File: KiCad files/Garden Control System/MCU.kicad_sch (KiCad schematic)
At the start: 24 parts, among them SW1 SW_SPDT, U1 STM32F207ZGTx, Y1 16MHz

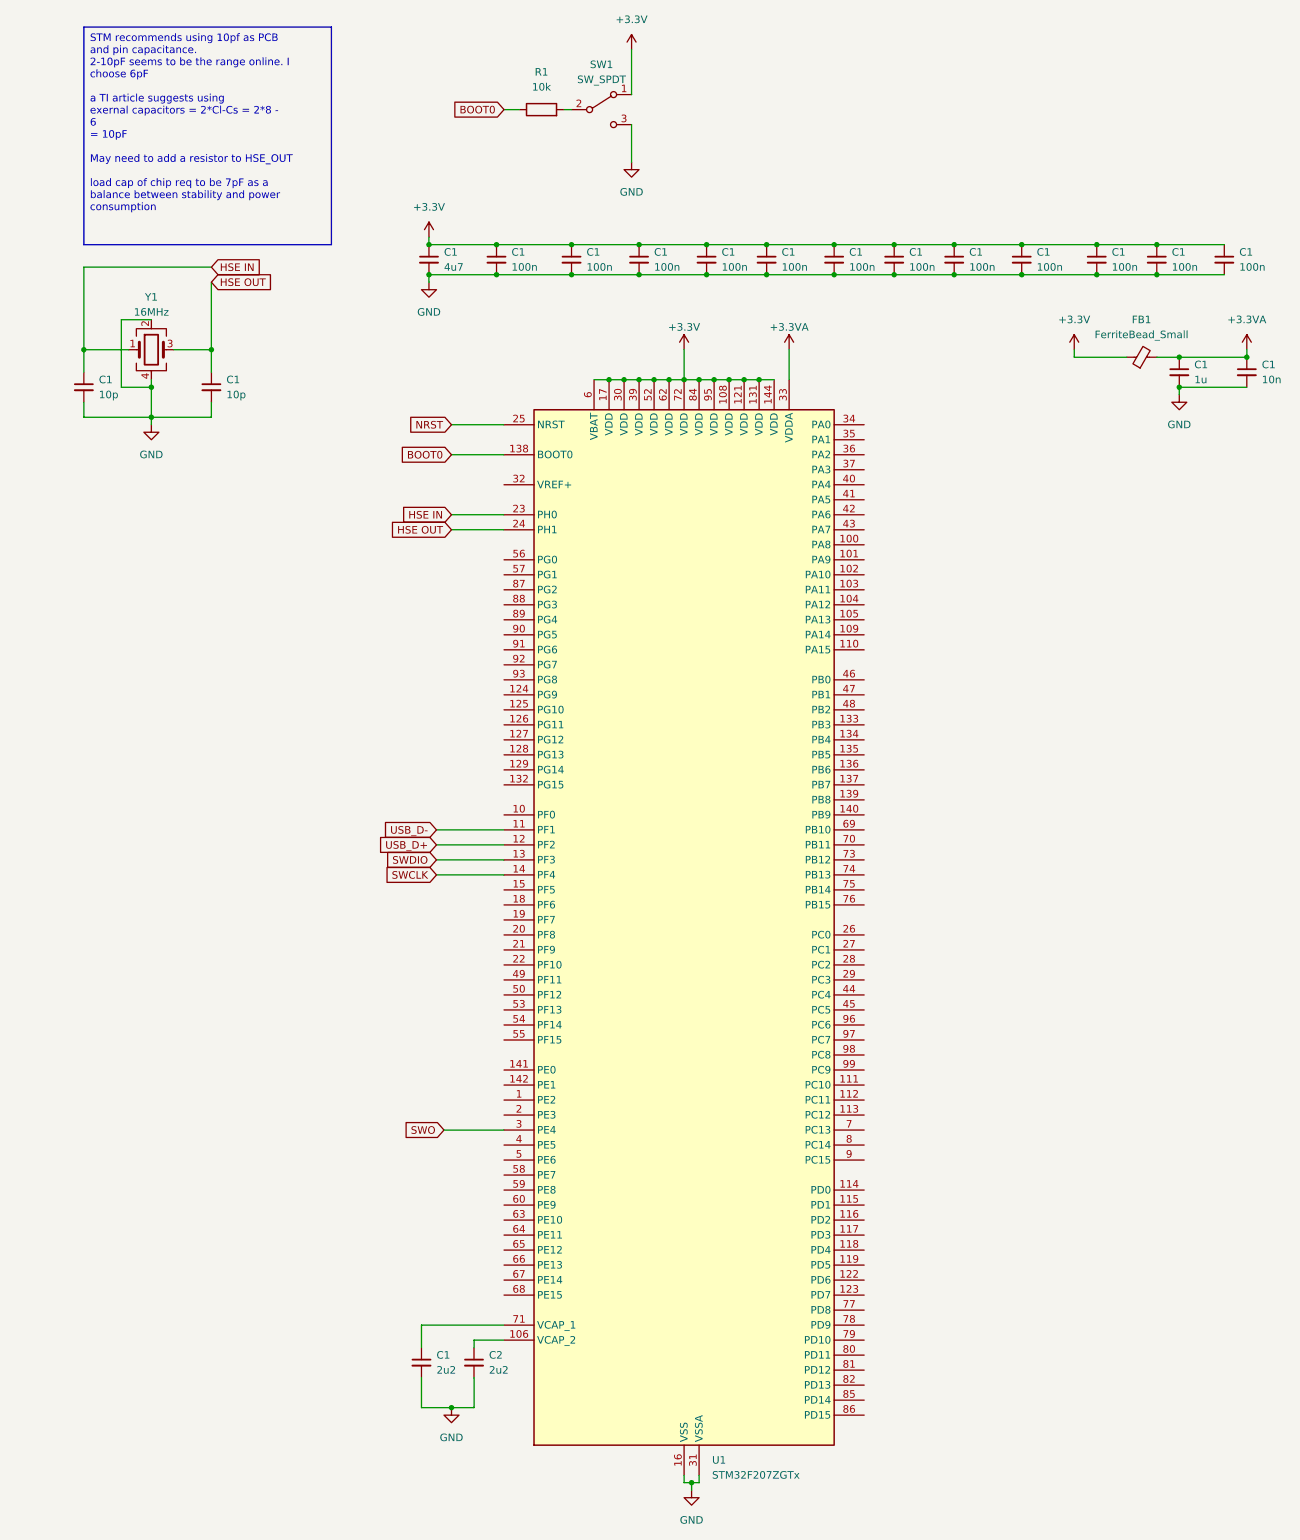
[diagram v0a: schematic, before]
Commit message: Close to finishing ethernet side
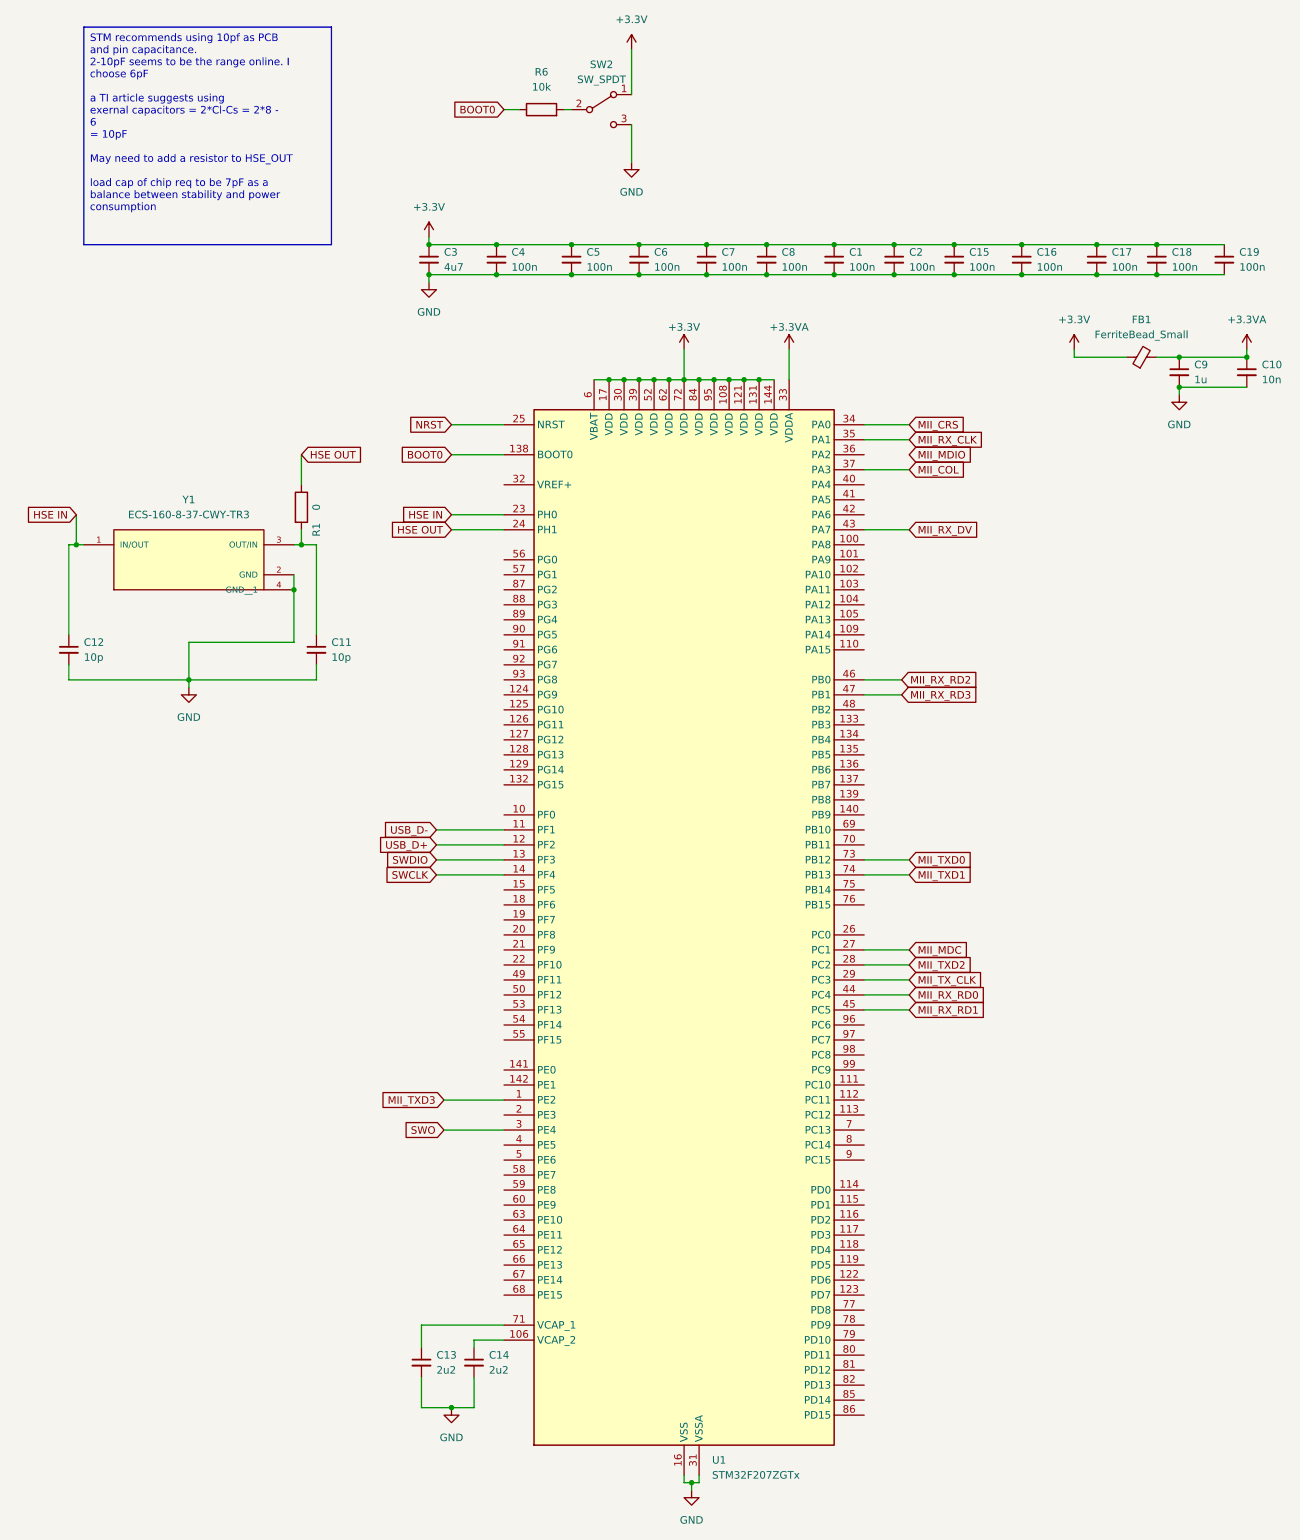
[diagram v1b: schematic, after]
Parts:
- removed Y1: 16MHz, symbol Device:Crystal_GND24
- added R1: 0, symbol Device:R
- added Y1: ECS-160-8-37-CWY-TR3, ECS-160-8-37-CWY-TR3:XTAL_ECS-160-8-37-CWY-TR3, symbol ECS-160-8-37-CWY-TR3:ECS-160-8-37-CWY-TR3
- renumbered C1 to C10, C1 to C11, C1 to C12, C1 to C13, C2 to C14, C1 to C15, C1 to C16, C1 to C17, C1 to C18, C1 to C19, C1 to C2, C1 to C3, C1 to C4, C1 to C5, C1 to C6, C1 to C7, C1 to C8, C1 to C9, R1 to R6, SW1 to SW2
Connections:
- net GND: now also Y1.2 (GND), Y1.4 (GND__1)
- net HSE IN: now also Y1.1 (IN/OUT)
- net HSE OUT: now also R1.1; no longer C11.1
- net MII_TXD3: now reaches U1.1 (PE2)
- net MII_MDC: now reaches U1.27 (PC1)
- net MII_TXD2: now reaches U1.28 (PC2)
- net MII_TX_CLK: now reaches U1.29 (PC3)
- net MII_CRS: now reaches U1.34 (PA0)
- net MII_RX_CLK: now reaches U1.35 (PA1)
- net MII_COL: now reaches U1.37 (PA3)
- net MII_RX_DV: now reaches U1.43 (PA7)
- net MII_RX_RD0: now reaches U1.44 (PC4)
- net MII_RX_RD1: now reaches U1.45 (PC5)
- net MII_RX_RD2: now reaches U1.46 (PB0)
- net MII_RX_RD3: now reaches U1.47 (PB1)
- net MII_TXD0: now reaches U1.73 (PB12)
- net MII_TXD1: now reaches U1.74 (PB13)
- new net: C11.1, R1.2, Y1.3 (OUT/IN)
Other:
- moved on the sheet: C11, C12

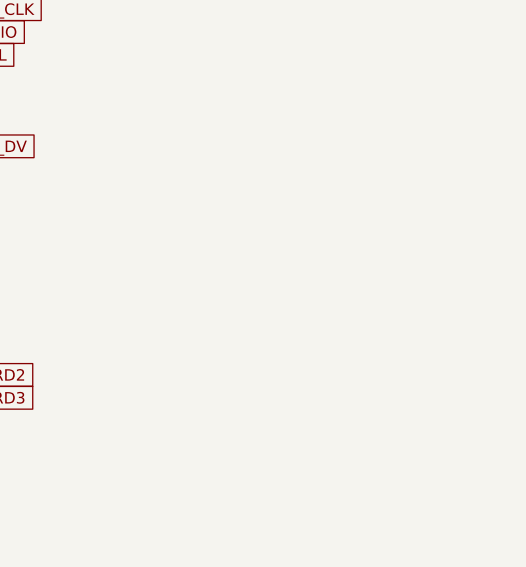
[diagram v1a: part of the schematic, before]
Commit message: working on power arch
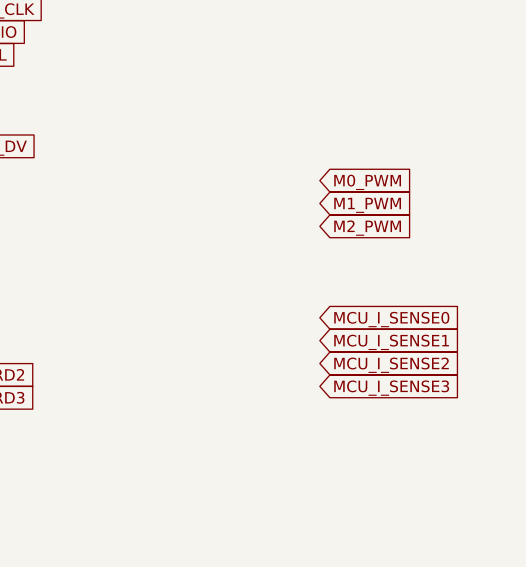
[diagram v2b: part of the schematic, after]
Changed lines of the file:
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@@
+		)
+	)
+	(global_label "MCU_I_SENSE0"
+		(shape input)
+		(at 207.01 124.46 0)
+		(fields_autoplaced yes)
+		(effects
+			(font
+				(size 1.27 1.27)
+			)
+			(justify left)
+		)
+		(property "Intersheetrefs" "${INTERSHEET_REFS}"
+			(at 223.8441 124.46 0)
+			(effects
+				(font
+					(size 1.27 1.27)
+				)
+				(justify left)
+				(hide yes)
+			)
 		)
 	)
@@
 		)
 	)
+	(global_label "MCU_I_SENSE2"
+		(shape input)
+		(at 207.01 129.54 0)
+		(fields_autoplaced yes)
+		(effects
+			(font
+				(size 1.27 1.27)
+			)
+			(justify left)
+		)
+		(property "Intersheetrefs" "${INTERSHEET_REFS}"
+			(at 223.8441 129.54 0)
+			(effects
+				(font
+					(size 1.27 1.27)
+				)
+				(justify left)
+				(hide yes)
+			)
+		)
+	)
+	(global_label "M1_PWM"
+		(shape input)
+		(at 207.01 111.76 0)
+		(fields_autoplaced yes)
+		(effects
+			(font
+				(size 1.27 1.27)
+			)
+			(justify left)
+		)
+		(property "Intersheetrefs" "${INTERSHEET_REFS}"
+			(at 217.7965 111.76 0)
+			(effects
+				(font
+					(size 1.27 1.27)
+				)
+				(justify left)
+				(hide yes)
+			)
+		)
+	)
 	(global_label "MII_RX_RD2"
 		(shape input)
@@
 		)
 	)
+	(global_label "M0_PWM"
+		(shape input)
+		(at 207.01 109.22 0)
+		(fields_autoplaced yes)
+		(effects
+			(font
+				(size 1.27 1.27)
+			)
+			(justify left)
+		)
+		(property "Intersheetrefs" "${INTERSHEET_REFS}"
+			(at 217.7965 109.22 0)
+			(effects
+				(font
+					(size 1.27 1.27)
+				)
+				(justify left)
+				(hide yes)
+			)
+		)
+	)
 	(global_label "HSE OUT"
 		(shape input)
@@
 			(effects
 				(font
+					(size 1.27 1.27)
+				)
+				(justify left)
+				(hide yes)
+			)
+		)
+	)
+	(global_label "MCU_I_SENSE3"
+		(shape input)
+		(at 207.01 132.08 0)
+		(fields_autoplaced yes)
+		(effects
+			(font
+				(size 1.27 1.27)
+			)
+			(justify left)
+		)
+		(property "Intersheetrefs" "${INTERSHEET_REFS}"
+			(at 223.8441 132.08 0)
+			(effects
+				(font
+					(size 1.27 1.27)
+				)
+				(justify left)
+				(hide yes)
+			)
+		)
+	)
+	(global_label "M2_PWM"
+		(shape input)
+		(at 207.01 114.3 0)
+		(fields_autoplaced yes)
+		(effects
+			(font
+				(size 1.27 1.27)
+			)
+			(justify left)
+		)
+		(property "Intersheetrefs" "${INTERSHEET_REFS}"
+			(at 217.7965 114.3 0)
+			(effects
+				(font
+					(size 1.27 1.27)
+				)
+				(justify left)
+				(hide yes)
+			)
+		)
+	)
+	(global_label "MCU_I_SENSE1"
+		(shape input)
+		(at 207.01 127 0)
+		(fields_autoplaced yes)
+		(effects
+			(font
+				(size 1.27 1.27)
+			)
+			(justify left)
+		)
+		(property "Intersheetrefs" "${INTERSHEET_REFS}"
+			(at 223.8441 127 0)
+			(effects
+				(font
